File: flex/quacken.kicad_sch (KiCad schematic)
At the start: 99 parts, among them J1 CIRQUE_Left, J2 CIRQUE_Right, J3 USB_C_Receptacle_USB2.0_16P, U1 W25Q128JVS, U2 RP2040, U3 PCAL6524HEAZ, U4 XC6206PxxxMR, U5 SRV05-4, Y1 12MHz 18pF

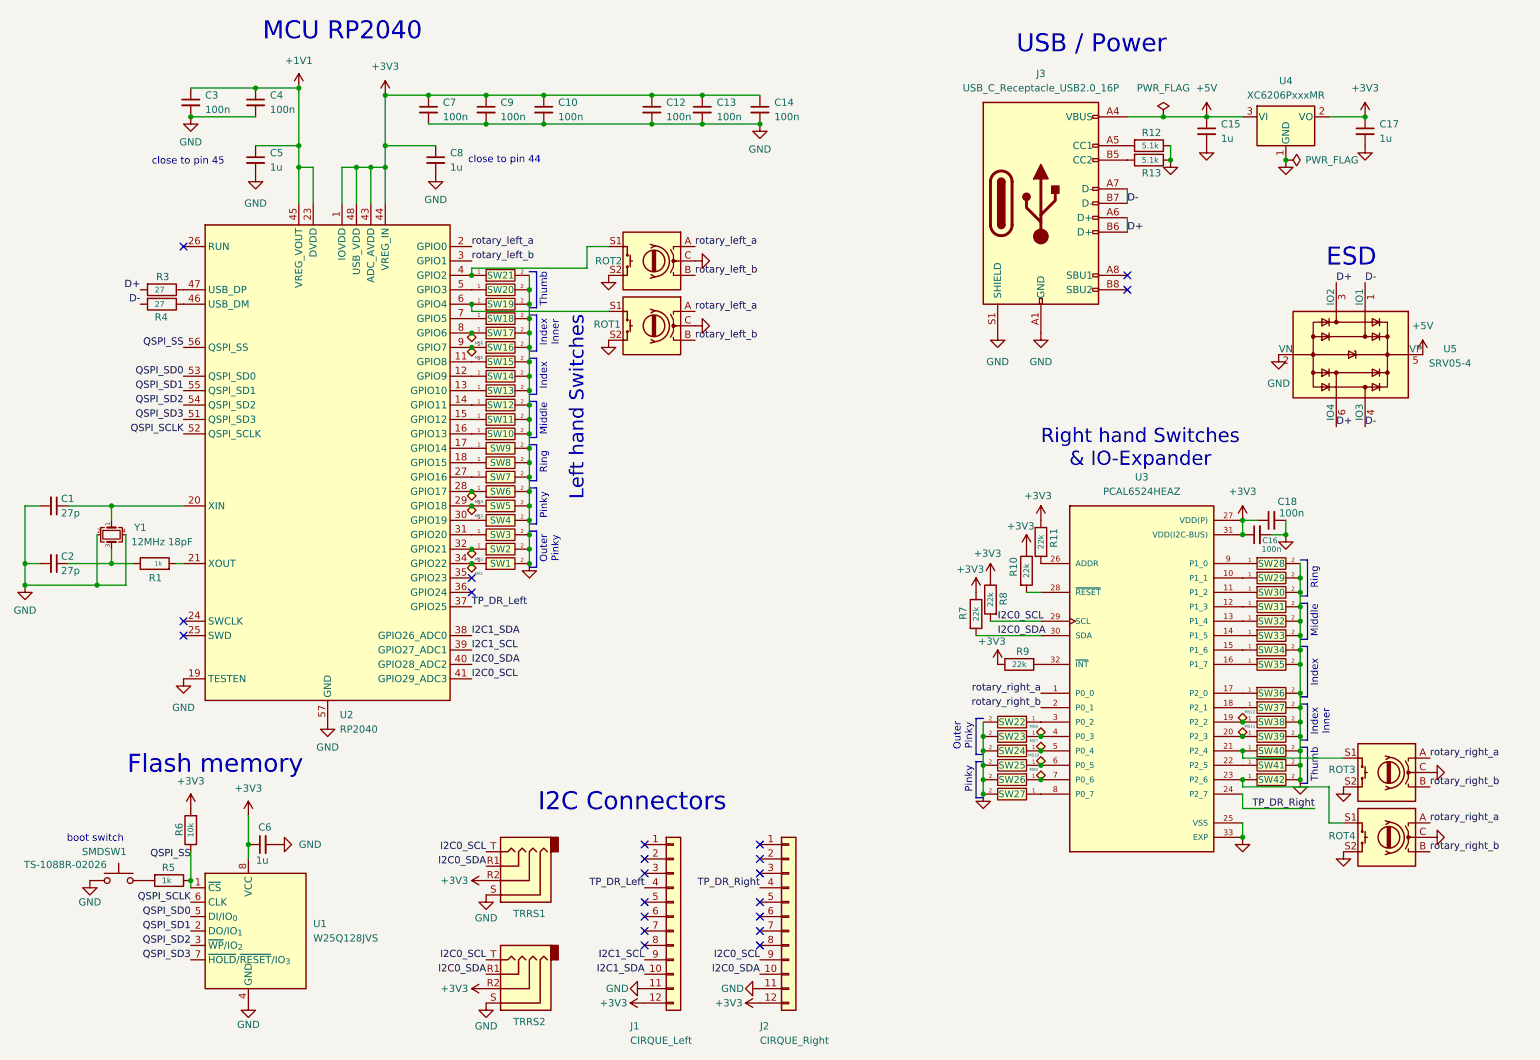
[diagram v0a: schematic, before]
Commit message: flex 25.11 (#11)
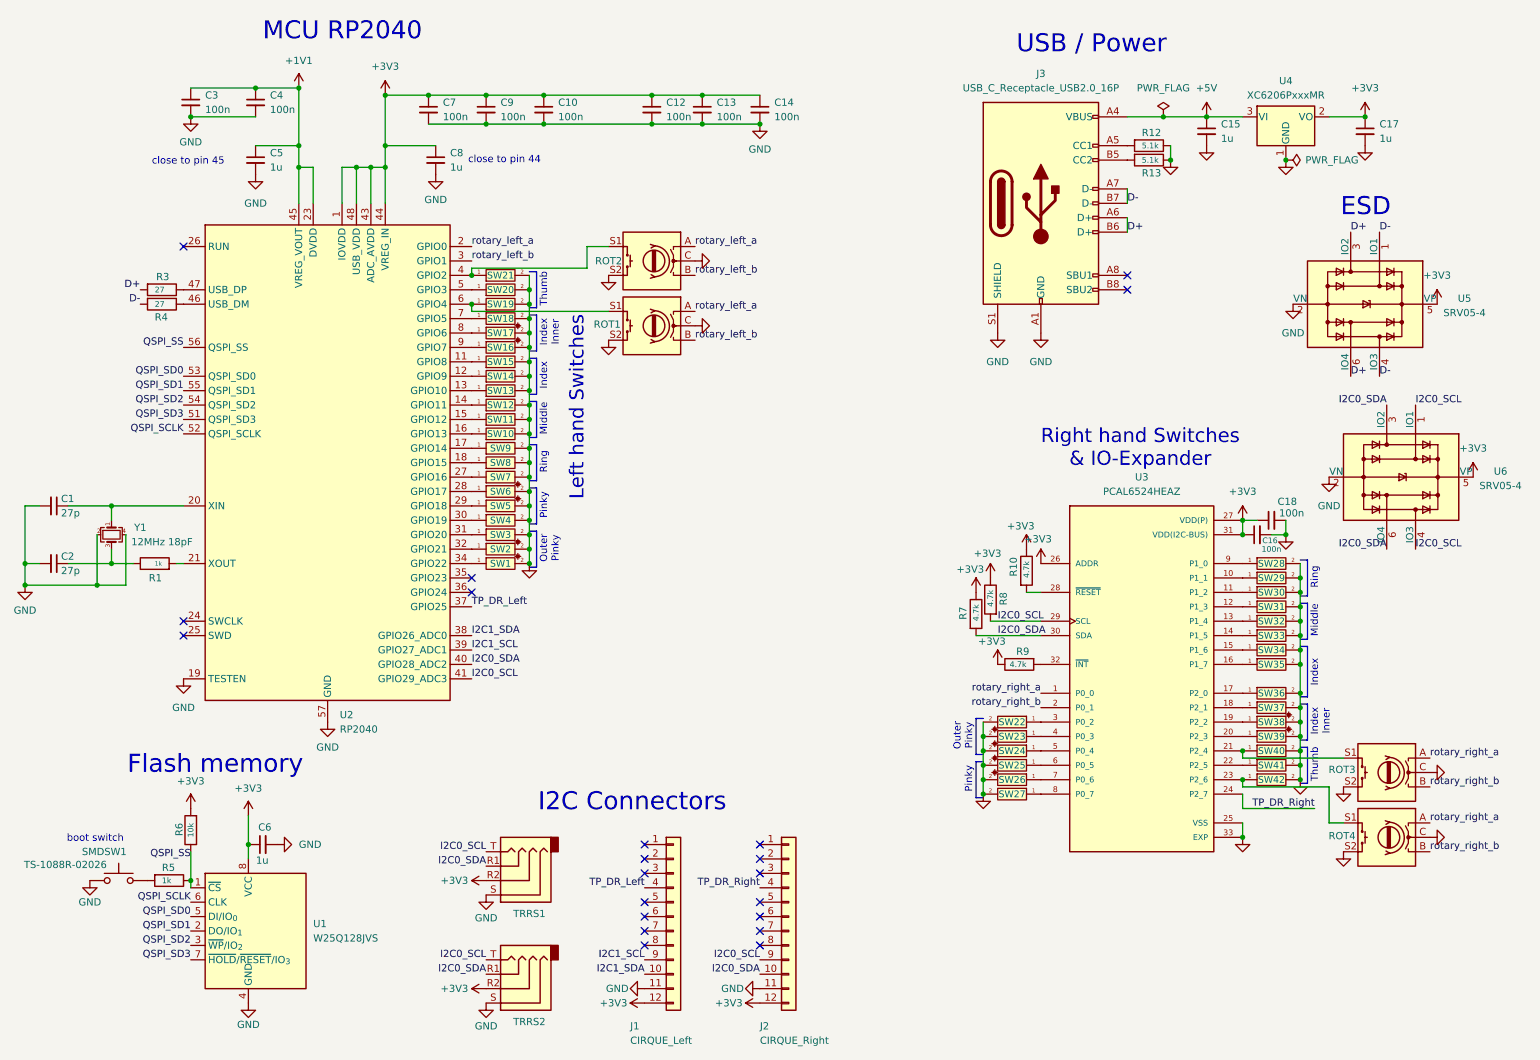
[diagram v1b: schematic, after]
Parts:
- removed MS1, MS10, MS11, MS12, MS2, MS3, MS4, MS5, MS6, MS7, MS8, MS9: ~, keyboard:MedianPosition, symbol Keyboards:MedianSwitch
- removed R11: 22k, Resistor_SMD:R_0402_1005Metric, symbol Device:R
- added U6: SRV05-4, Package_TO_SOT_SMD:SOT-23-6, symbol Power_Protection:SRV05-4
- R10, R7, R8, R9: value 22k -> 4.7k
- SW1, SW16, SW17, SW2, SW23, SW24, SW25, SW26, SW38, SW39, SW5, SW6: footprint keyboard:PG1350 -> keyboard:Choc_Switch_Median; symbol Keyboards:Switch -> Keyboards:MedianSwitch
- SW10, SW11, SW12, SW13, SW14, SW15, SW18, SW19, SW20, SW21, SW22, SW27, SW28, SW29, SW3, SW30, SW31, SW32, SW33, SW34, SW35, SW36, SW37, SW4, SW40, SW41, SW42, SW7, SW8, SW9: footprint keyboard:PG1350 -> keyboard:Choc_Switch
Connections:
- net +3V3: now also U3.26 (ADDR), U5.5 (VP), U6.5 (VP)
- net +5V: no longer U5.5 (VP)
- net GND: now also U6.2 (VN)
- net I2C0_SCL: now also U6.1 (IO1), U6.4 (IO3)
- net I2C0_SDA: now also U6.3 (IO2), U6.6 (IO4)
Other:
- moved on the sheet: U5
